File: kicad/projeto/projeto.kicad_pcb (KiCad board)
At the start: 2 copper layers, 40 parts, among them Q1 BTA16-600B, Q2 BTA16-600B, U1 ESP-12E, U3v3 LM1117-3.3

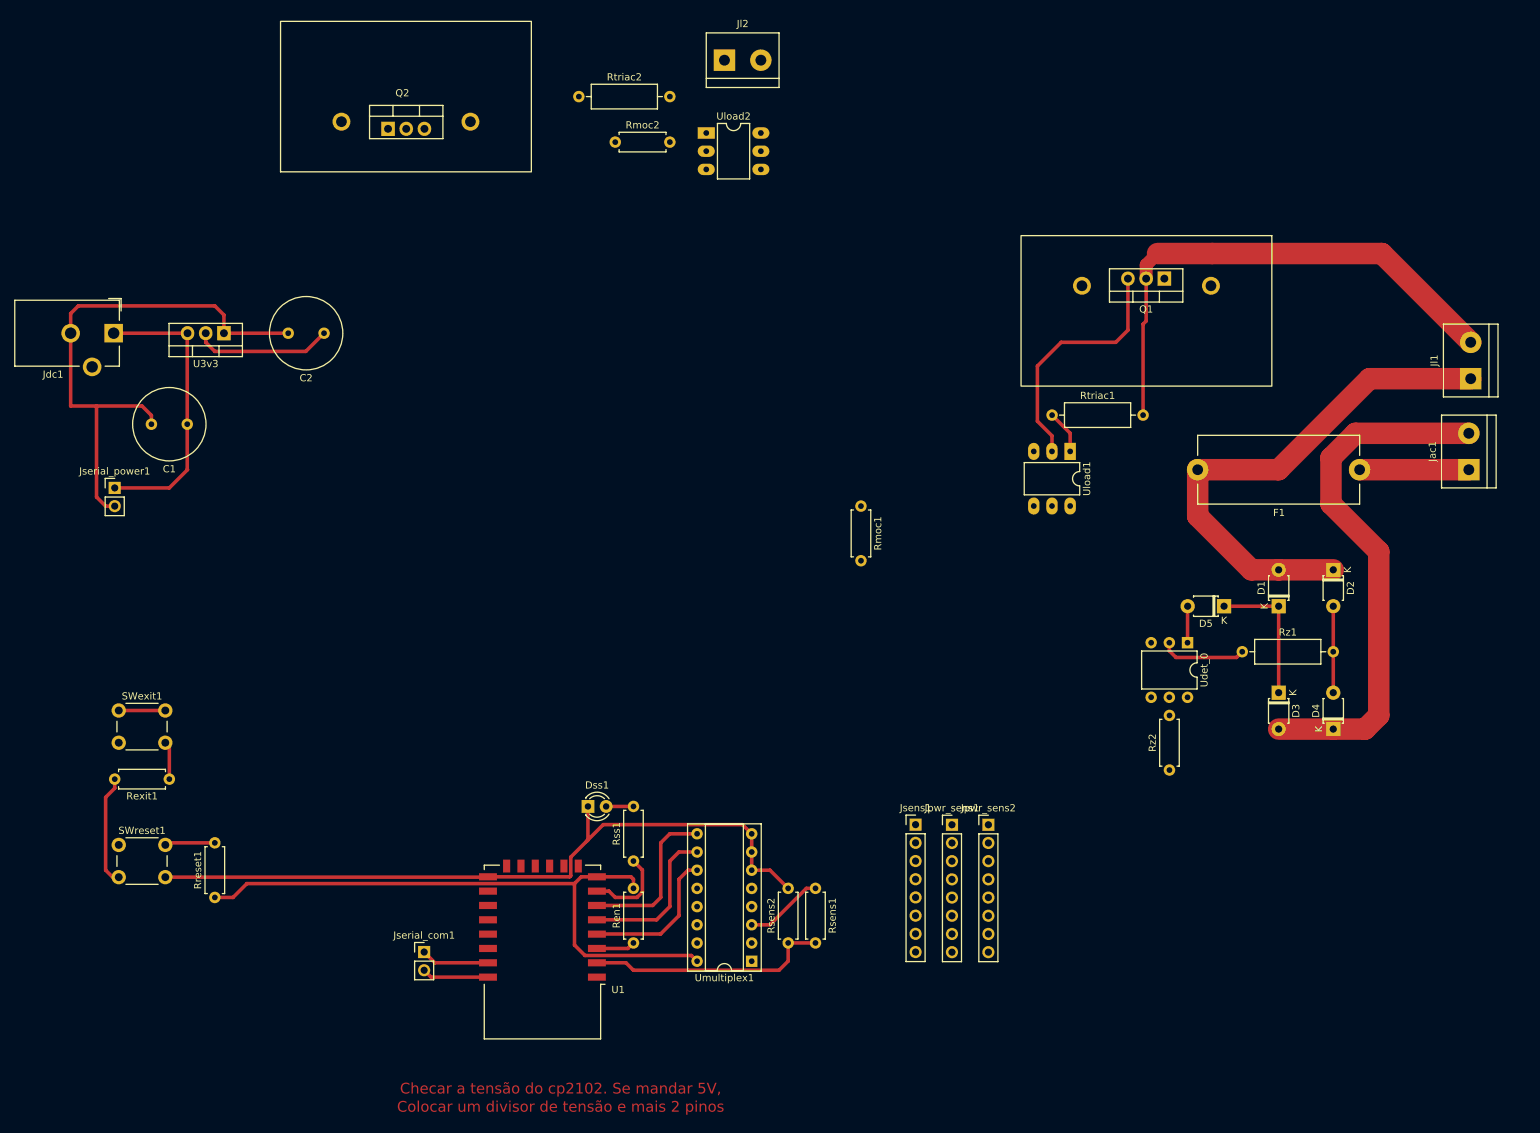
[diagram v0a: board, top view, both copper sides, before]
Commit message: Fazendo a PCB
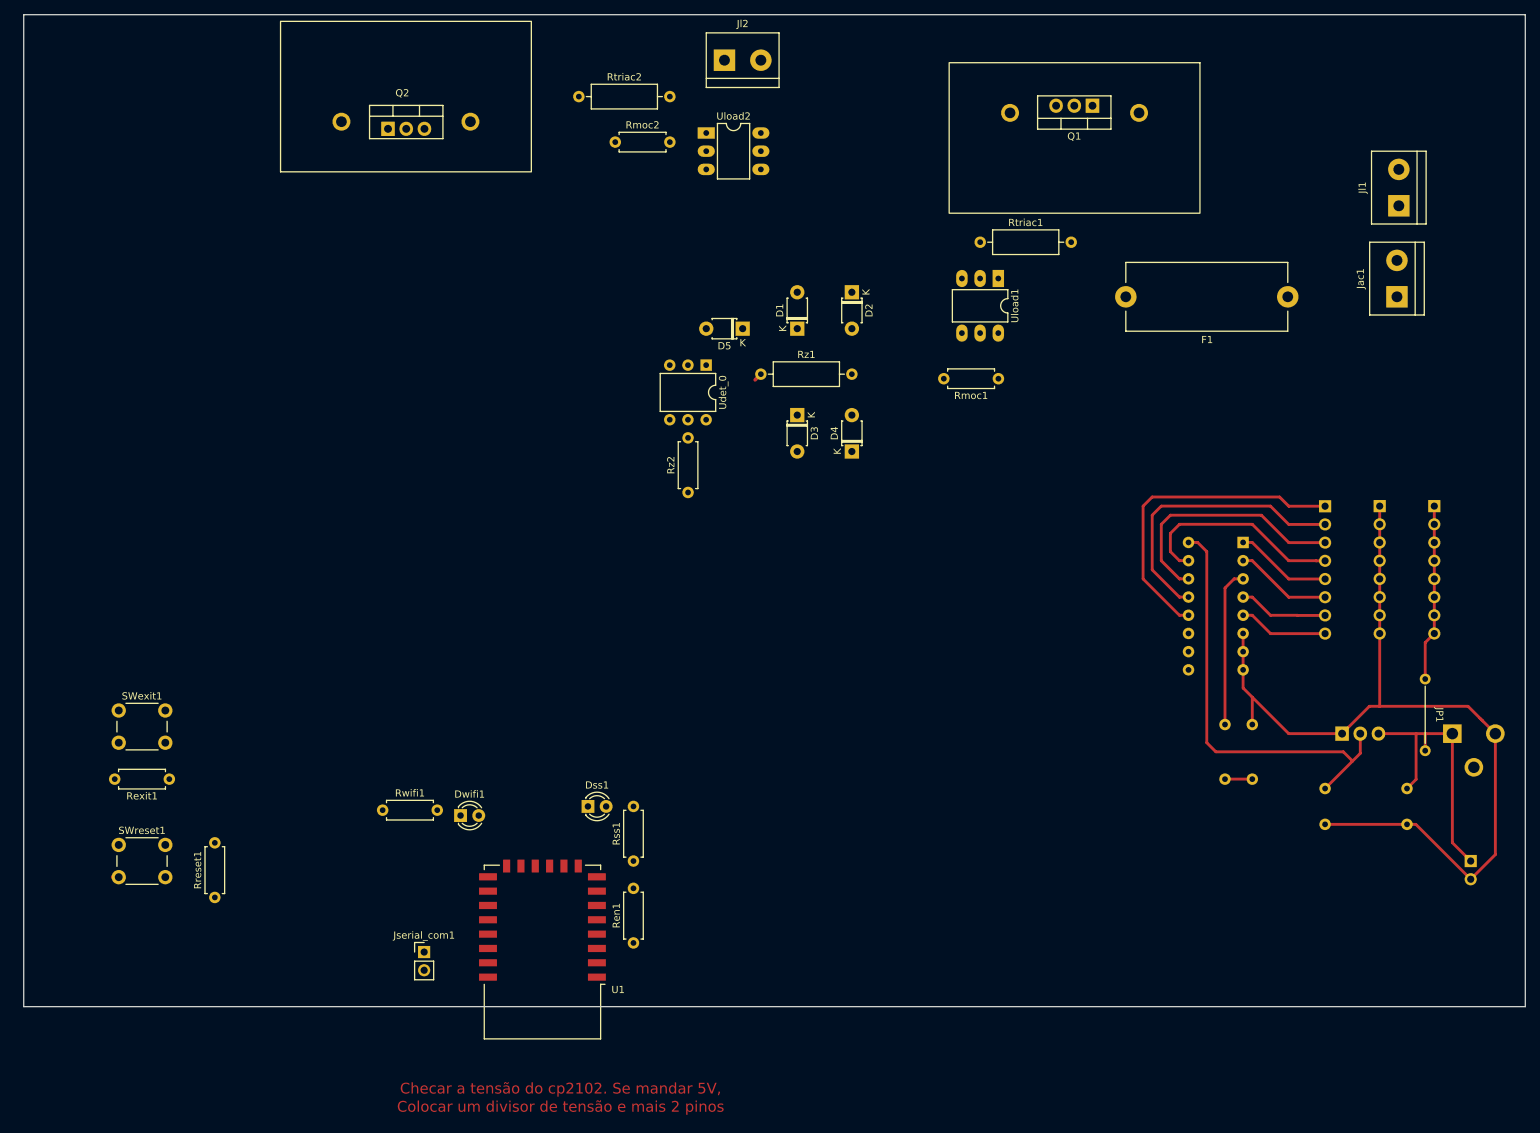
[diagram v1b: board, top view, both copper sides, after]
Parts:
- added Dwifi1: LED, LED_THT:LED_D3.0mm, F.Cu at (94.0, 125.7)
- added JP1: Jumper_2_Bridged, Jumper:jumper_10mm, F.Cu at (228.6, 106.7)
- added Rwifi1: 260, Resistor_THT:R_Axial_DIN0207_L6.3mm_D2.5mm_P7.62mm_Horizontal, F.Cu at (83.1, 125.0)
- C1, C2, Jdc1, Jpwr_sens1, Jpwr_sens2, Jsens1, Jserial_power1, Rsens1, Rsens2, U3v3, Umultiplex1: moved to B.Cu
- moved Jserial_power1 196.3 mm to (234.9, 132.1), turned to 180 degrees
- moved Jdc1 195.0 mm to (232.4, 114.3)
- moved C1 177.7 mm to (226.1, 122.0), turned to -90 degrees
- moved U3v3 165.7 mm to (217.0, 114.3), turned to 0 degrees
- moved C2 153.5 mm to (214.6, 122.0), turned to -90 degrees
- moved Umultiplex1 90.1 mm to (203.2, 87.6)
- moved Jpwr_sens1 80.7 mm to (229.9, 82.5), turned to 180 degrees
- moved D1 77.5 mm to (141.0, 57.8)
- moved D2 77.5 mm to (148.6, 52.7)
- moved D3 77.5 mm to (141.0, 69.8)
- moved D4 77.5 mm to (148.6, 74.9)
- moved D5 77.5 mm to (133.3, 57.8)
- moved Rz1 77.5 mm to (135.9, 64.1)
- moved Rz2 77.5 mm to (125.7, 80.6)
- moved Udet_0 77.5 mm to (128.3, 62.9)
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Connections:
- net Net-(Jsens1-Pad5) renamed /S4
- Jpwr_sens1 pad 1: +5V -> Net-(JP1-Pad1)
- Jpwr_sens1 pad 2: +5V -> Net-(JP1-Pad1)
- Jpwr_sens1 pad 3: +5V -> Net-(JP1-Pad1)
- Jpwr_sens1 pad 4: +5V -> Net-(JP1-Pad1)
- Jpwr_sens1 pad 5: +5V -> Net-(JP1-Pad1)
- Jpwr_sens1 pad 6: +5V -> Net-(JP1-Pad1)
- Jpwr_sens1 pad 7: +5V -> Net-(JP1-Pad1)
- Jpwr_sens1 pad 8: +5V -> Net-(JP1-Pad1)
- Jsens1 pad 1: Net-(Jsens1-Pad1) -> /S3
- Jsens1 pad 2: Net-(Jsens1-Pad2) -> /S0
- Jsens1 pad 3: Net-(Jsens1-Pad3) -> /S1
- Jsens1 pad 4: Net-(Jsens1-Pad4) -> /S2
- Jsens1 pad 6: Net-(Jsens1-Pad6) -> /S6
- Jsens1 pad 7: Net-(Jsens1-Pad7) -> /S7
- Jsens1 pad 8: Net-(Jsens1-Pad8) -> /S5
- U1 pad 17: unconnected-(U1-Pad17) -> /wifi_status
- Umultiplex1 pad 12: Net-(Jsens1-Pad4) -> /S3
- Umultiplex1 pad 13: Net-(Jsens1-Pad1) -> /S0
- Umultiplex1 pad 14: Net-(Jsens1-Pad2) -> /S1
- Umultiplex1 pad 15: Net-(Jsens1-Pad3) -> /S2
- Umultiplex1 pad 2: Net-(Jsens1-Pad7) -> /S6
- Umultiplex1 pad 4: Net-(Jsens1-Pad8) -> /S7
- Umultiplex1 pad 5: Net-(Jsens1-Pad6) -> /S5
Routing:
- net /AC2: track 74.1 -> 0.00 mm
- net Net-(Jl1-Pad2): track 72.2 -> 0.00 mm
- net /AC1: track 71.9 -> 0.00 mm
- net GND: track 194.1 -> 127.0 mm
- net +3V3: track 113.5 -> 60.8 mm
- net /S3: track 0.00 -> 45.1 mm
- net /S0: track 0.00 -> 40.0 mm
- net /S1: track 0.00 -> 34.9 mm
- net Net-(Q1-Pad3): track 34.7 -> 0.00 mm
- net /multiplex_out: track 34.0 -> 3.81 mm
- net /S2: track 0.00 -> 29.8 mm
- net Net-(JP1-Pad1): track 0.00 -> 24.7 mm
- net /multiplex_C: track 22.6 -> 0.00 mm
- net /multiplex_B: track 21.6 -> 0.00 mm
- net /multiplex_A: track 20.7 -> 0.03 mm
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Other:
- board outline added: 209.5 x 138.4 mm
- board text added: "+5V"
- board text added: "gnd"
